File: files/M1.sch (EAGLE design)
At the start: 27 parts, among them U1 CR2032-BS-6-1

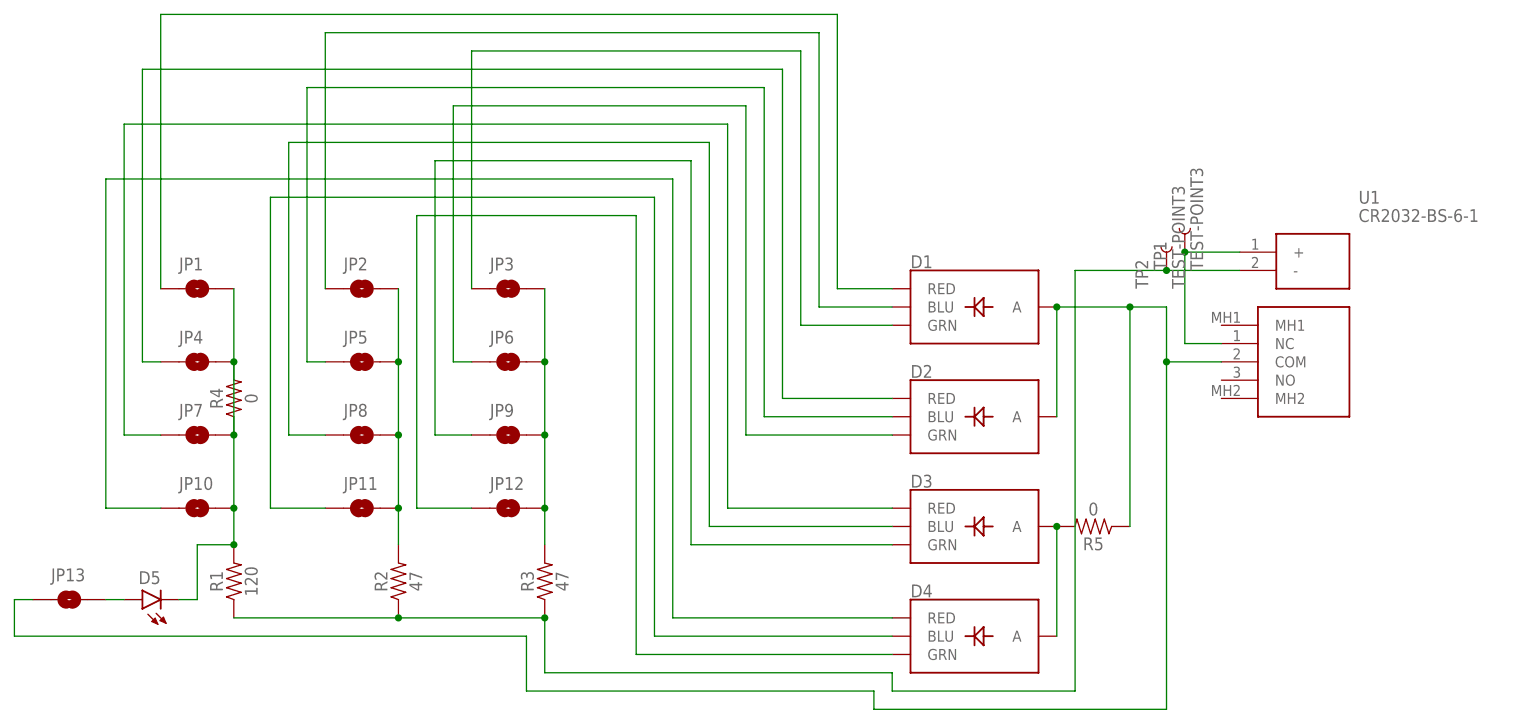
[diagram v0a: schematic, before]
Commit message: Update files to RC
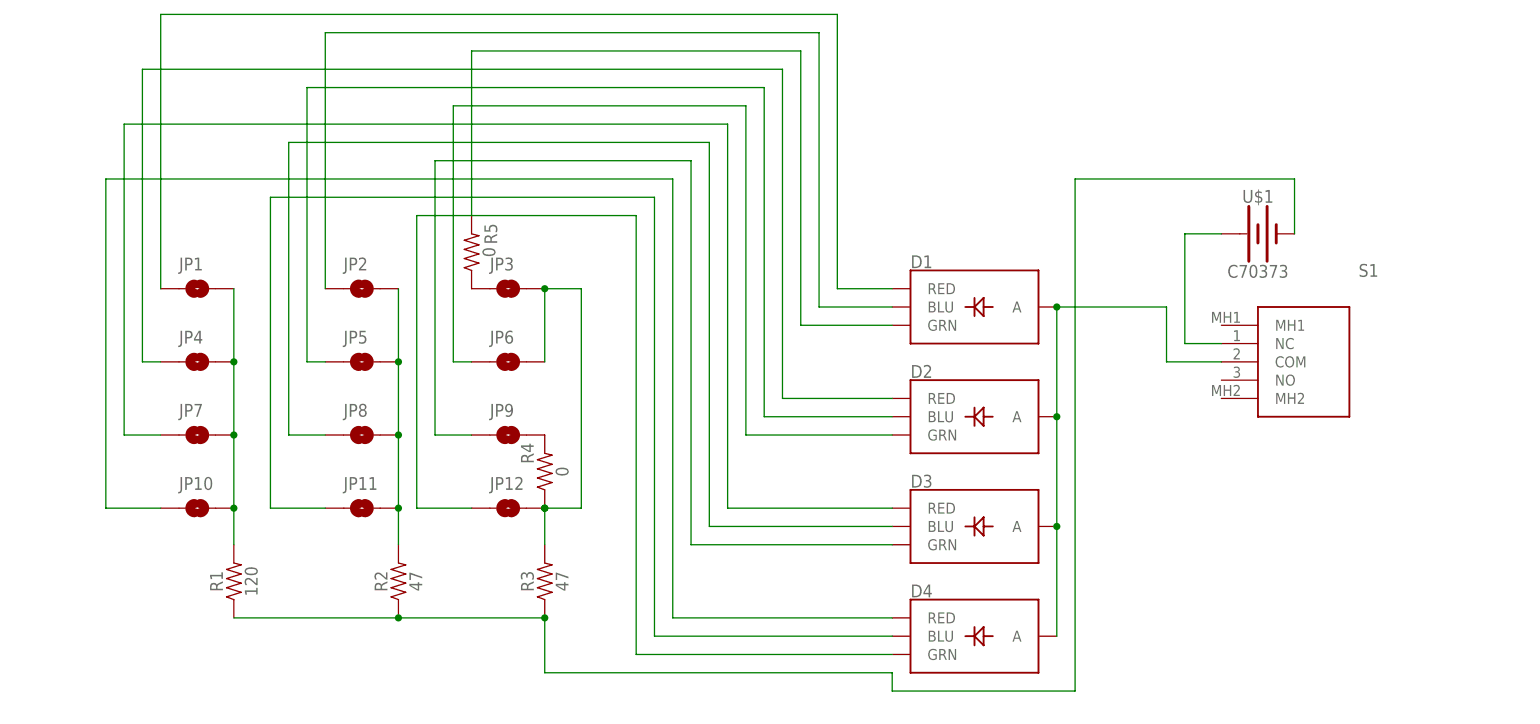
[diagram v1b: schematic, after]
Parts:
- removed D5: PWR, SparkFun-LED:LED-FKIT-1206
- removed JP13: JUMPER-SMT_2_NO_SILK, SparkFun-Jumpers:JUMPER-SMT_2_NO_SILK
- removed TP1, TP2: TEST-POINT3, SparkFun-Connectors:TEST-POINT3
- removed U1: CR2032-BS-6-1, CR2032-BS-6-1:CR2032-BS-6-1
- added U$1: C70373, untitled:C70373
- R1, R2, R3, R4, R5: device SparkFun-Resistors:RESISTOR1206 -> SparkFun-Resistors:RESISTOR0805
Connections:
- net N$1: now also D3.A, D4.A; no longer JP13.1, R5.1
- net N$16: no longer D5.C, R4.1, R4.2
- net N$17: now also R4.2; no longer JP12.2, JP3.2, JP6.2, R3.2
- net N$18: now also JP3.1, R5.1; no longer D3.A, D4.A, R5.2
- net N$2: now also U$1.+; no longer TP1.1, U1.+
- net N$25: now also U$1.-; no longer TP2.1, U1.-
- net N$4: now also JP12.2, JP3.2, JP6.2, R3.2, R4.1; no longer D5.A, JP13.2
- net N$6: now also R5.2; no longer JP3.1
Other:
- moved on the sheet: R4, R5
